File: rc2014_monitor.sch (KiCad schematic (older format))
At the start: 22 parts, among them J1 RC2014Pro, J3 USB_B_Micro, SW1 SW_Coded_Octal-8, U1 74HCT138, U2 74HCT151, U3 74HCT244, U4 74HCT244, U5 74HCT244, U6 74HCT32

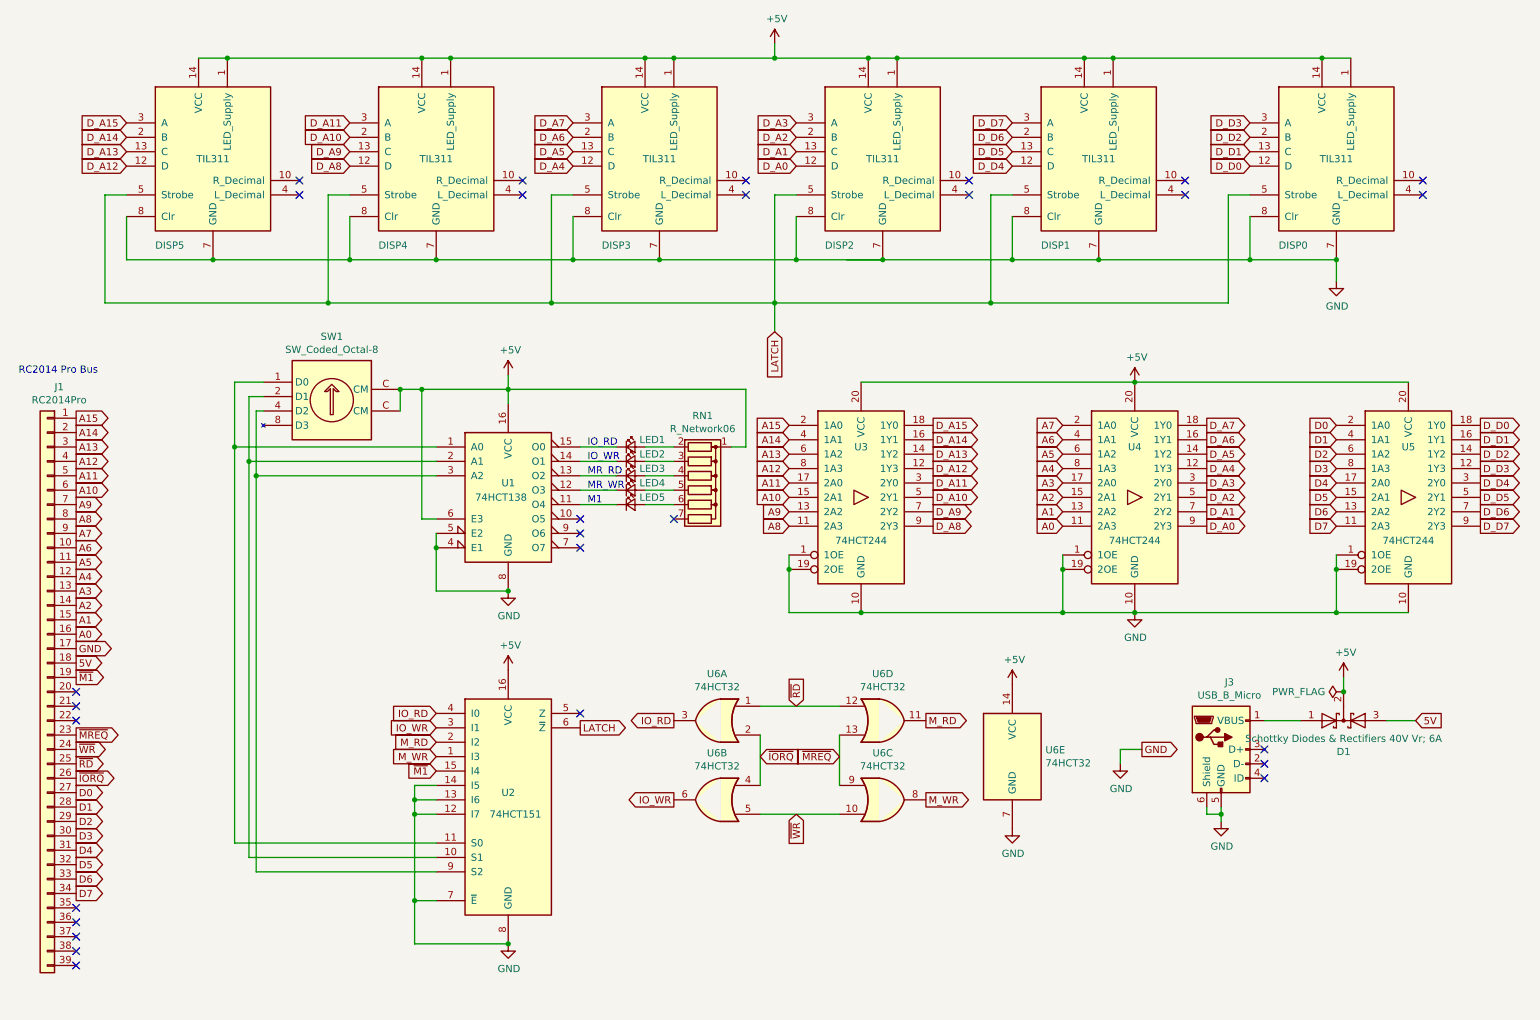
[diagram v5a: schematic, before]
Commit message: reorganized wiring
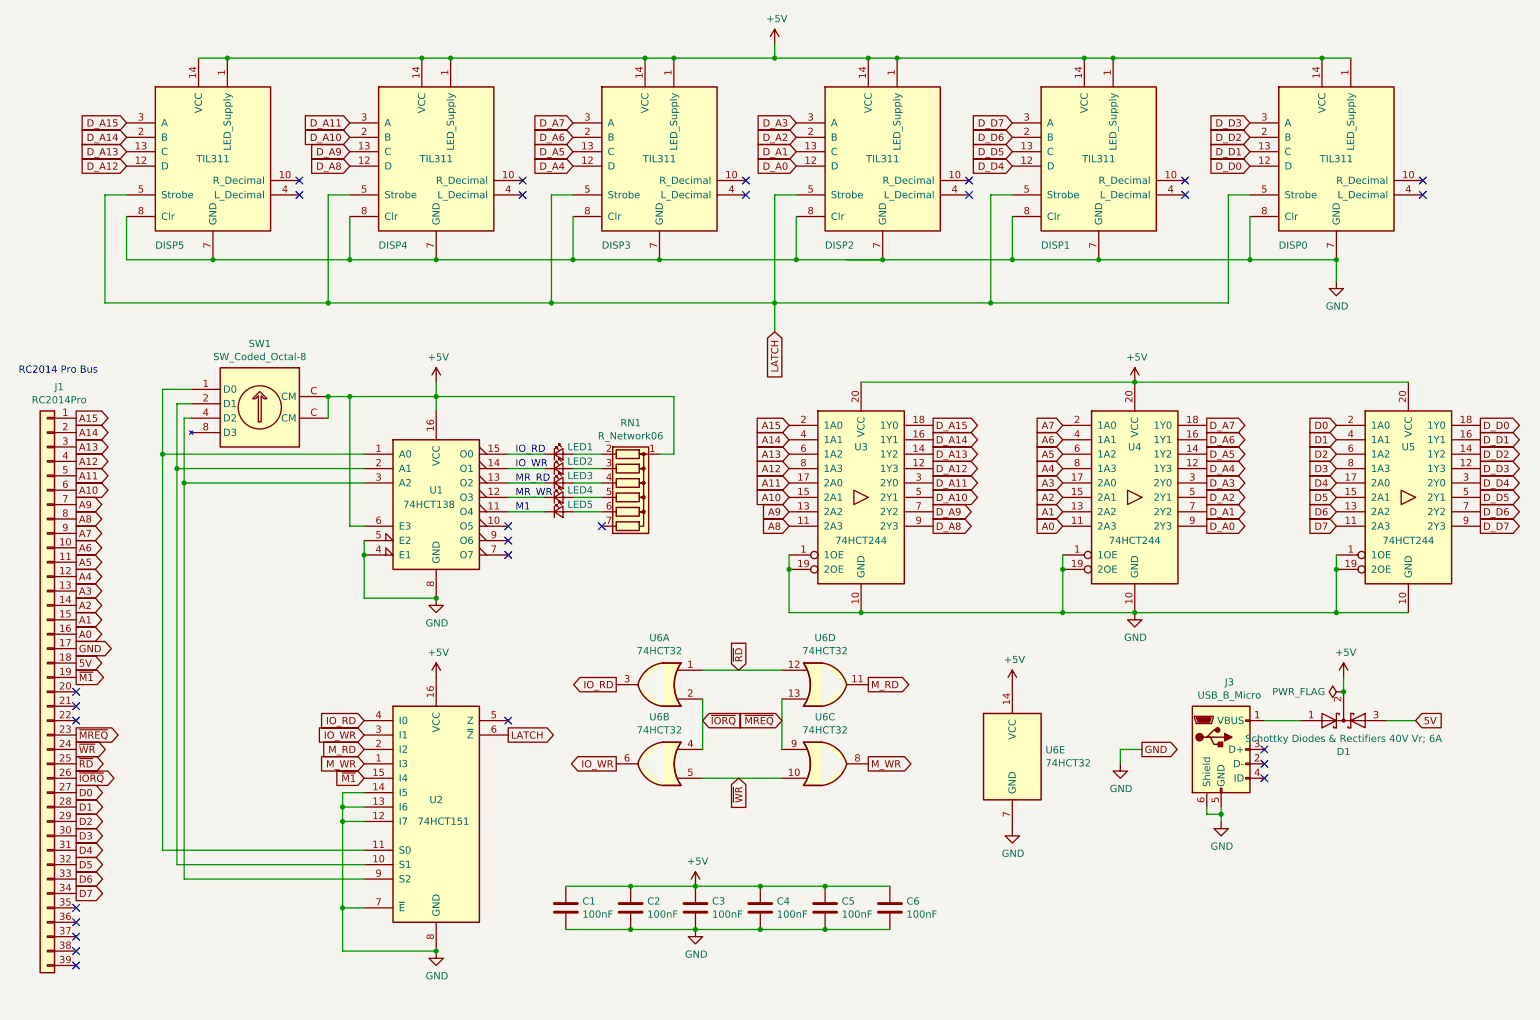
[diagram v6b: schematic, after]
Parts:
- added C1, C2, C3, C4, C5, C6: 100nF, Capacitor_THT:C_Disc_D5.0mm_W2.5mm_P2.50mm, symbol Device:C
- DISP0, DISP1, DISP2, DISP3, DISP5: footprint Package_DIP:DIP-14_W7.62mm_Socket_LongPads -> Package_DIP:DIP-14_W7.62mm_Socket
- DISP4: footprint Package_DIP:DIP-14_W7.62mm_Socket_LongPads -> Package_DIP:DIP-14_W7.62mm
- U1, U2: footprint Package_DIP:DIP-16_W7.62mm_LongPads -> Package_DIP:DIP-16_W7.62mm
- U3, U4, U5: footprint Package_DIP:DIP-20_W7.62mm_Socket_LongPads -> Package_DIP:DIP-20_W7.62mm_Socket
- U6: footprint Package_DIP:DIP-14_W7.62mm_LongPads -> Package_DIP:DIP-14_W7.62mm
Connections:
- net +5V: now also C1.1, C2.1, C3.1, C4.1, C5.1, C6.1
- net GND: now also C1.2, C2.2, C3.2, C4.2, C5.2, C6.2
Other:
- moved on the sheet: LED1, LED2, LED3, LED4, LED5, RN1, SW1, U1, U2, U6A, U6B, U6C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
